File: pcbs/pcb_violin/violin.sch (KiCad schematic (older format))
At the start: 38 parts

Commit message: PCB update power pins
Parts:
- added J?: Screw_Terminal_01x02, symbol Connector:Screw_Terminal_01x02
- added J?: Conn_02x05_Odd_Even, symbol Connector_Generic:Conn_02x05_Odd_Even
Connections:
- net +3V3: now also J?.1 (Pin_1)
- net +9V: now also J?.1 (Pin_1)
- net GND: now also J?.2 (Pin_2), J?.3 (Pin_3), J?.5 (Pin_5), J?.9 (Pin_9)
- net NRST: now also J?.10 (Pin_10)
- net SWCLK: now also J?.4 (Pin_4)
- net SWO: now also J?.6 (Pin_6)
- net I2C1_SDA: now reaches U?.59 (PB7)
- net I2C1_SCL: now reaches U?.61 (PB8)
- net SWIDO renamed SWDIO
- net SWDIO: now also J?.2 (Pin_2)
- no-connect marks 2 -> 4
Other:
- moved on the sheet: C?, J?, L?, R?, U?

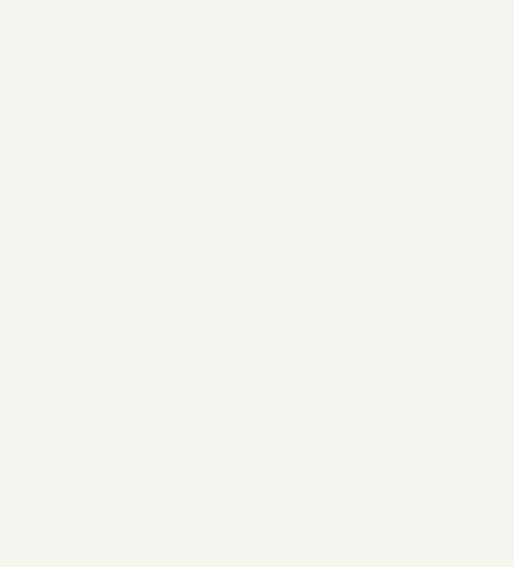
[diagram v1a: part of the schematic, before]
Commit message: Considering MAX604 LDO Voltage Regulator
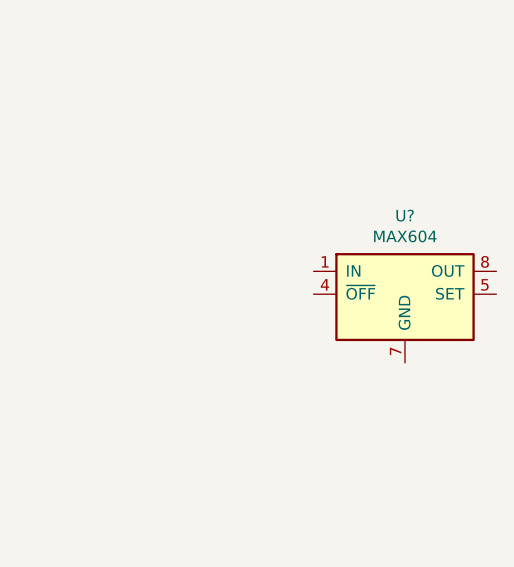
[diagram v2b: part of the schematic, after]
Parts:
- added U?: MAX604, symbol Regulator_Linear:MAX604
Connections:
- new net: U?.2 (GND), U?.3 (GND), U?.6 (GND), U?.7 (GND)
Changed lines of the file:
@@
 Text GLabel 5800 4100 2    50   Input ~ 0
 I2C1_SDA
+$Comp
+L Regulator_Linear:MAX604 U?
+U 1 1 60DEFDA8
+P 22050 -2050
+F 0 "U?" H 22050 -1708 50  0000 C CNN
+F 1 "MAX604" H 22050 -1799 50  0000 C CNN
+F 2 "" H 22050 -1725 50  0001 C CIN
+F 3 "http://datasheets.maximintegrated.com/en/ds/MAX603-MAX604.pdf" H 22050 -2100 50  0001 C CNN
+	1    22050 -2050
+	1    0    0    -1
+$EndComp
 $EndSCHEMATC
